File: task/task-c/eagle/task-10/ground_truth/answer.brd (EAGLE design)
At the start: 54.3 x 38.1 mm, 12 parts, among them IC1 16F84, U1 78L05

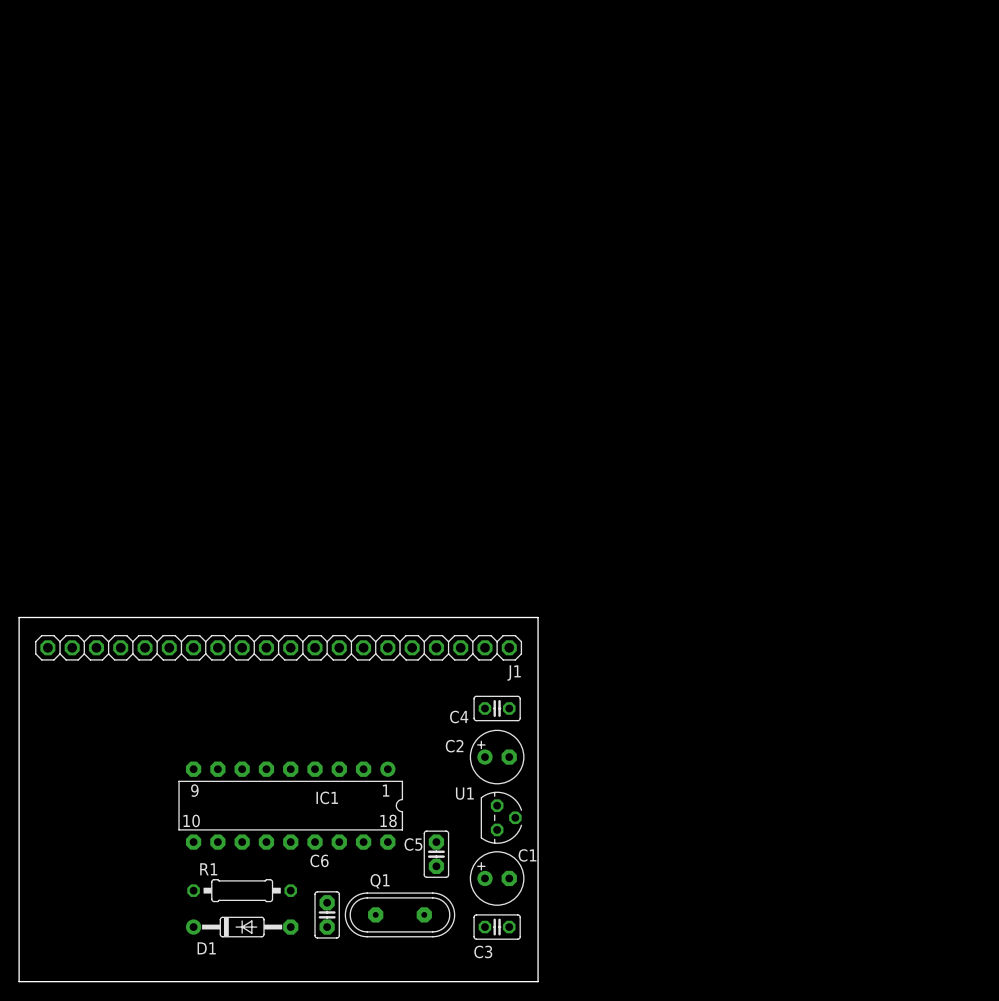
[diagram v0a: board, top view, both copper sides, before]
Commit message: Refine engineering task metadata and instructions
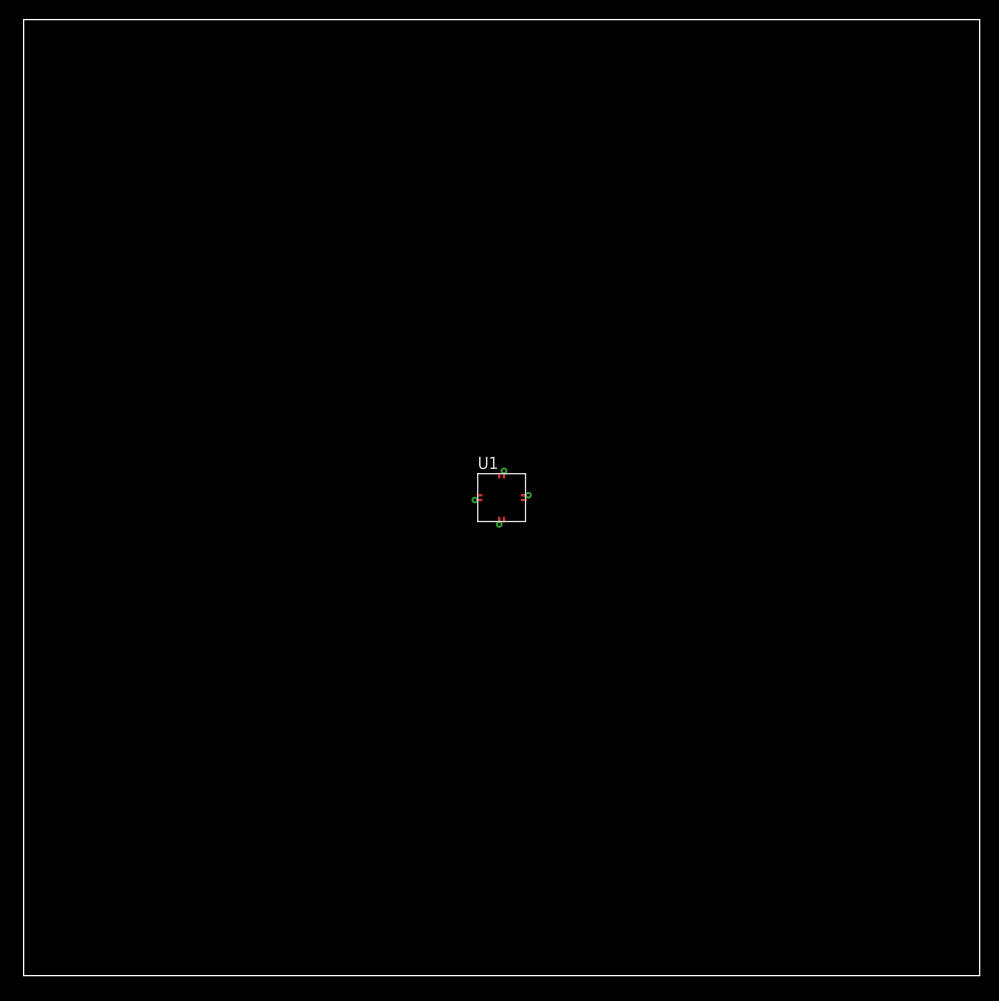
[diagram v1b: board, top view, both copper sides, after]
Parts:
- removed C1, C2: 10u, polcap:E2,5-6
- removed C3, C4: 10n, rcl:C025-025X050
- removed C5, C6: 27p, capacitor-wima:C2,5-2
- removed D1: 1N4148, diode:DO35-10
- removed IC1: 16F84, microchip:DIL18
- removed J1: (no value), PINHEAD:1X20
- removed Q1: (no value), special:QS
- removed R1: 2.2k, rcl:0207/10
- U1: value 78L05 -> (none); device linear:TO92 -> synth:QFN8
- moved U1 33.5 mm to (50.0, 50.0), turned to 0 degrees
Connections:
- removed net +12V: C1.+, C3.2, J1.2, U1.3
- removed net A0: IC1.17, J1.4
- removed net A1: IC1.18, J1.5
- removed net A2: IC1.1, J1.6
- removed net A3: IC1.2, J1.7
- removed net A4: IC1.3, J1.8
- removed net B0: IC1.6, J1.9
- removed net B1: IC1.7, J1.10
- removed net B2: IC1.8, J1.11
- removed net B3: IC1.9, J1.12
- removed net B4: IC1.10, J1.13
- removed net B5: IC1.11, J1.14
- removed net B6: IC1.12, J1.15, J1.18
- removed net B7: IC1.13, J1.16, J1.17
- removed net GND: C1.-, C2.-, C3.1, C4.1, C5.1, C6.1, IC1.5, J1.1, J1.20, U1.2
- removed net N$2: D1.A, R1.1
- removed net N$4: C6.2, IC1.15, Q1.1
- removed net VCC: C2.+, C4.2, IC1.14, J1.3, R1.2, U1.1
- new net N$5: U1.5
- new net N$7: U1.7
- net N$1: now also U1.1; no longer D1.K, IC1.4, J1.19
- net N$3: now also U1.3; no longer C5.2, IC1.16, Q1.2
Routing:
- net N$7: track 0.00 -> 0.50 mm, vias 0 -> 1
- net N$5: track 0.00 -> 0.50 mm, vias 0 -> 1
- net N$3: track 0.00 -> 0.50 mm, vias 0 -> 1
- net N$1: track 0.00 -> 0.50 mm, vias 0 -> 1
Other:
- board size 54.3 x 38.1 mm -> 100 x 100 mm
